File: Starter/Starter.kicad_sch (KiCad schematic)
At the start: 61 parts, among them J2 Speaker, J3 UART1, J5 Conn_01x08_Pin, J7 DACOUT, SW1 UP, SW2 LEFT, SW3 DOWN, SW4 RIGHT, U1 MPU-6050, U2 LP-MSPM0G3507, U3 MCP34119D, U4 HiLetGo_ST7735R, U5 ULN2003B, U6 TSOP31438

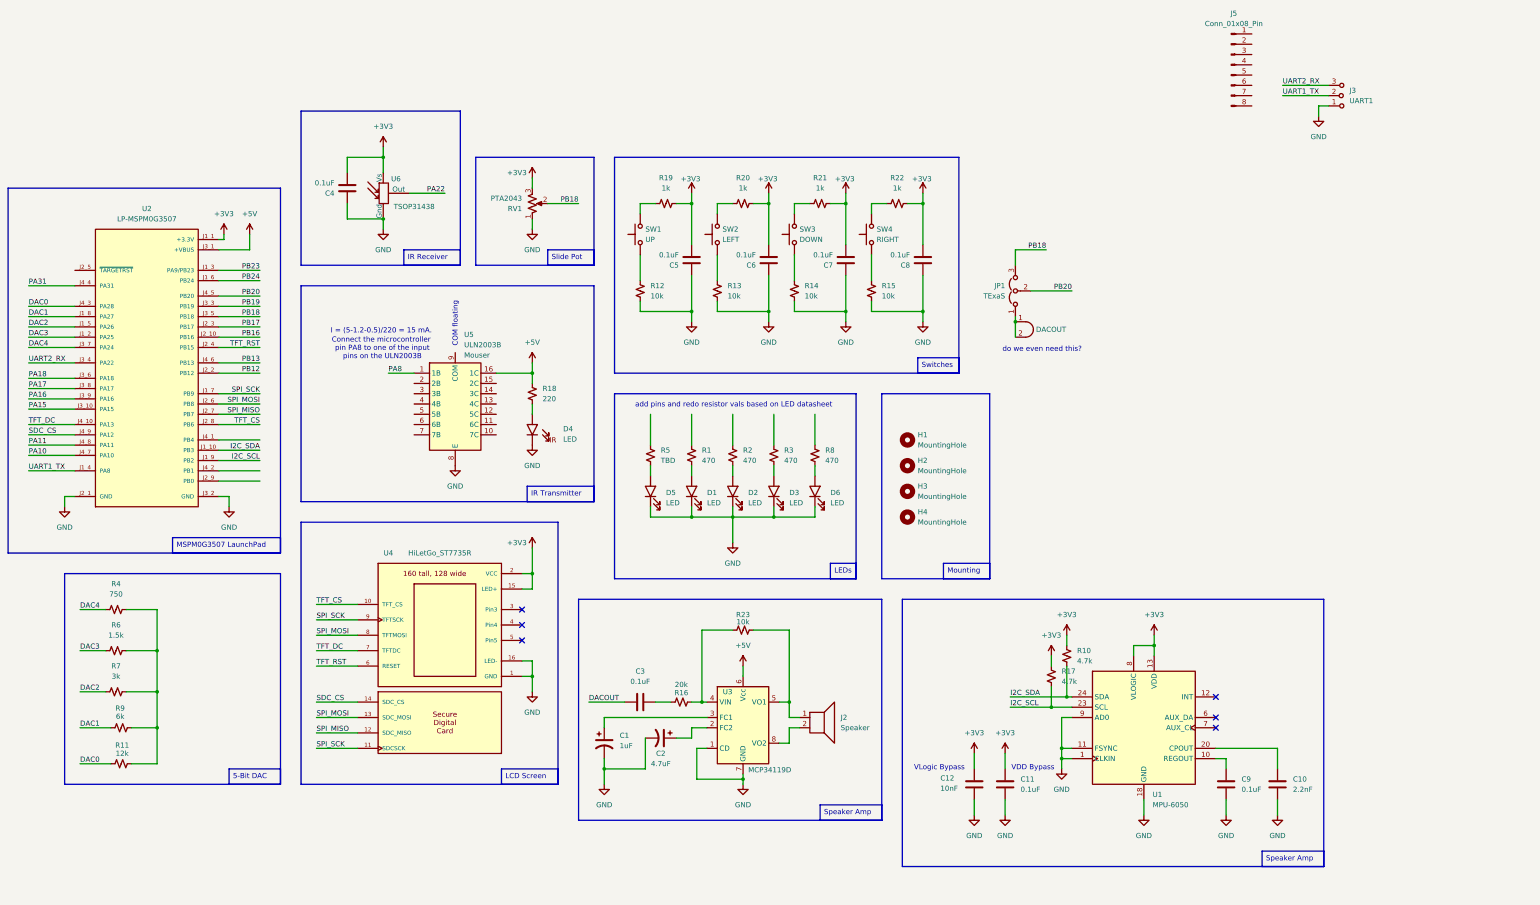
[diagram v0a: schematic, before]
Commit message: wow im dumb
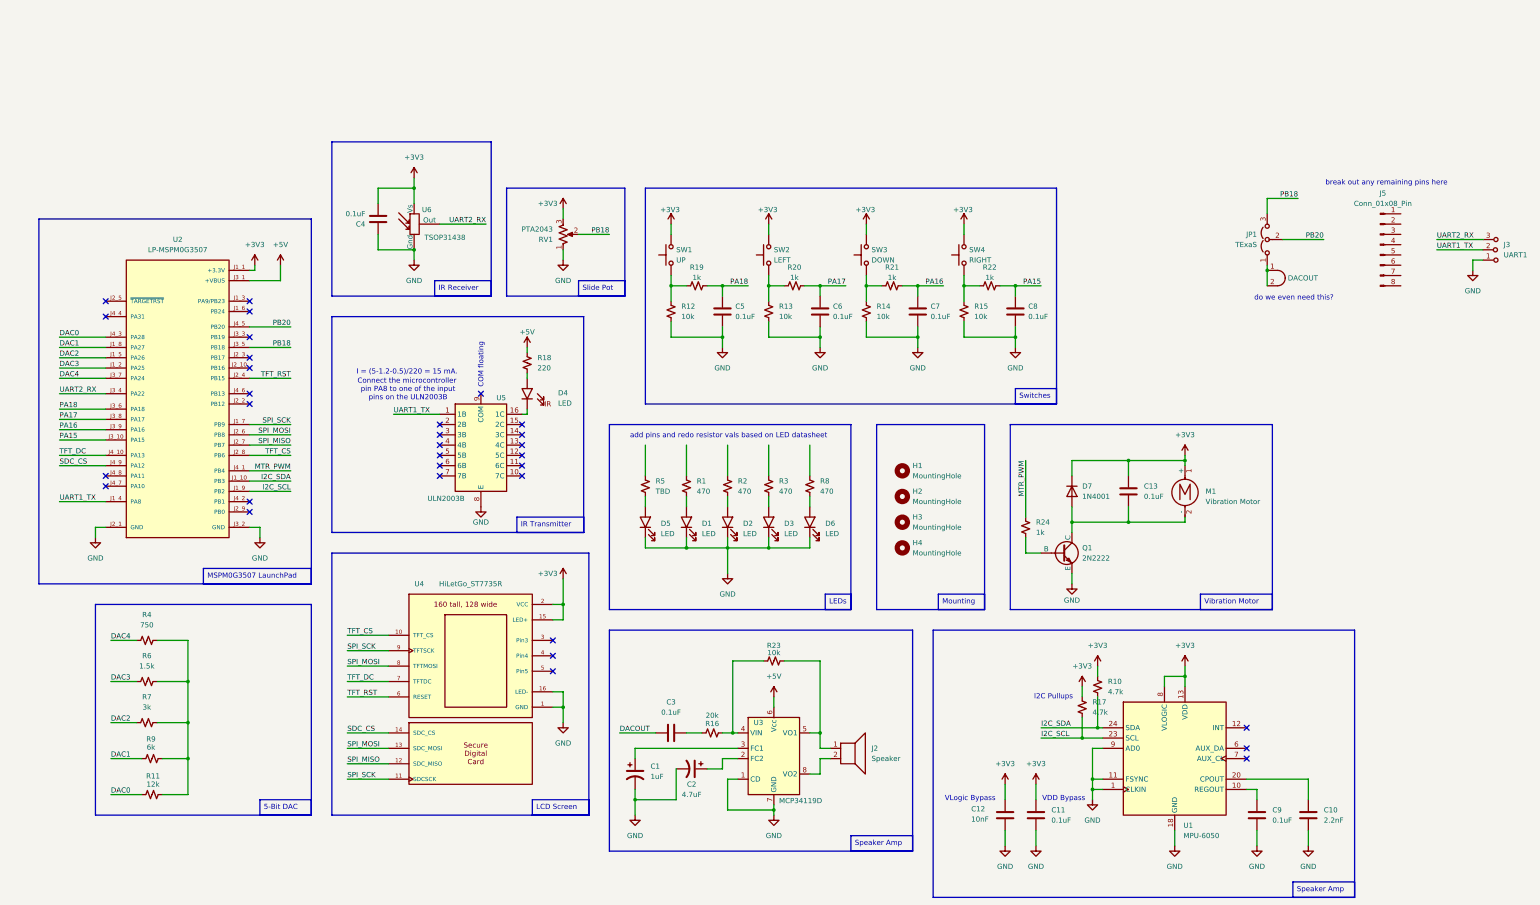
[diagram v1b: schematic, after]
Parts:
- added C13: 0.1uF, ECE319K:C_Axial_200mil, symbol ECE319H:C
- added D7: 1N4001, Diode_THT:D_DO-41_SOD81_P10.16mm_Horizontal, symbol Diode:1N4001
- added M1: Vibration Motor, symbol Motor:Motor_DC
- added Q1: 2N2222, symbol Simulation_SPICE:NPN
- added R24: 1k, ECE319K:R_Axial_DIN0204_L3.6mm_D1.6mm_P7.62mm_Horizontal, symbol ECE319K:R_0.125W
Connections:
- net PA22 is gone; now on net UART2_RX: U6.3 (Out)
- net PA8 is gone; now on net UART1_TX: U5.1 (1B)
- net +3V3: now also SW1.2, SW2.2, SW3.2, SW4.2, C13.1, D7.1 (K), M1.1 (+); no longer C5.2, C6.2, C7.2, C8.2, R19.1, R20.1, R21.1, R22.1
- net +5V: no longer U5.16 (1C)
- net GND: now also C5.2, C6.2, C7.2, C8.2, Q1.3 (E); no longer C5.1, C6.1, C7.1, C8.1, D4.1 (K)
- net PA15: now also C8.1, R22.1
- net PA16: now also C7.1, R21.1
- net PA17: now also C6.1, R20.1
- net PA18: now also C5.1, R19.1
- net at R13.1, SW2.1: now also R20.2
- net at R19.2: now also R12.1, SW1.1; no longer SW1.2
- net MTR_PWM: now reaches U2.J4_1 (PB4)
- net MTR_PWM: now also R24.1
- net at R21.2: now also R14.1, SW3.1; no longer SW3.2
- net at R15.1, SW4.1: now also R22.2
- net PA10: no longer names the net of U2.J4_7 (PA10)
- net PA11: no longer names the net of U2.J4_8 (PA11)
- net PA31: no longer names the net of U2.J4_4 (PA31)
- net PB12: no longer names the net of U2.J2_2 (PB12)
- net PB13: no longer names the net of U2.J4_6 (PB13)
- net PB16: no longer names the net of U2.J2_10 (PB16)
- net PB17: no longer names the net of U2.J2_3 (PB17)
- net PB19: no longer names the net of U2.J3_3 (PB19)
- net PB23: no longer names the net of U2.J1_3 (PA9/PB23)
- net PB24: no longer names the net of U2.J1_6 (PB24)
- new net: Q1.2 (B), R24.2
- new net: C13.2, D7.2 (A), M1.2 (-), Q1.1 (C)
- new net: D4.1 (K), U5.16 (1C)
- no-connect marks 6 -> 32
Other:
- note added: "I2C Pullups"
- note added: "break out any remaining pins here"
- moved on the sheet: C1, C10, C11, C12, C2, C3, C4, C5, C9, D1, D2, D3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
